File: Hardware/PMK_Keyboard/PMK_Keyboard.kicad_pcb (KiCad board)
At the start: 2 copper layers, 172 x 152 mm, 52 parts, among them IC1 SN74HC165PWR, IC2 SN74HC165PWR, IC3 SN74HC165PWR, IC4 SN74HC165PWR, IC5 SN74HC165PWR, IC7 ESP32-S2FH4, SW1 SW_Push, SW10 SW_Push, SW11 SW_Push, SW12 SW_Push, SW13 SW_Push, SW14 SW_Push, SW15 SW_Push, SW16 SW_Push, SW17 SW_Push, SW18 SW_Push, SW19 SW_Push, SW2 SW_Push, SW20 SW_Push, SW21 SW_Push, SW22 SW_Push, SW23 SW_Push, SW24 SW_Push, SW25 SW_Push, SW26 SW_Push, SW27 SW_Push, SW28 SW_Push, SW29 SW_Push, SW3 SW_Push, SW30 SW_Push, SW31 SW_Push, SW32 SW_Push, SW33 SW_Push, SW34 SW_Push, SW35 SW_Push, SW36 SW_Push, SW37 SW_Push, SW38 SW_Push, SW39 SW_Push, SW4 SW_Push, SW40 SW_Push, SW5 SW_Push, SW6 SW_Push, SW7 SW_Push, SW8 SW_Push, SW9 SW_Push

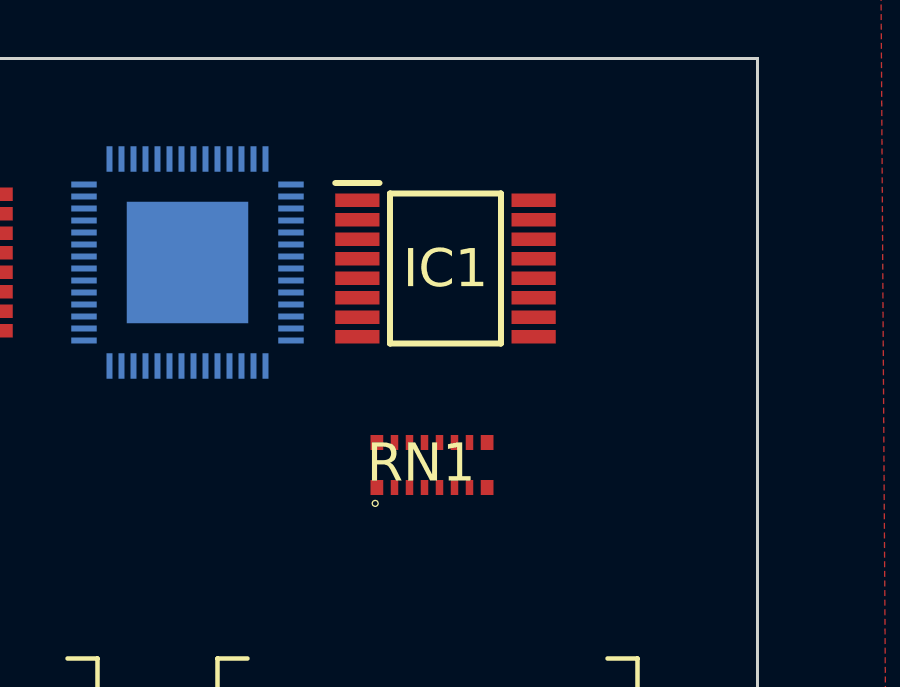
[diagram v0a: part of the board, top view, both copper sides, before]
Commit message: quick routing test
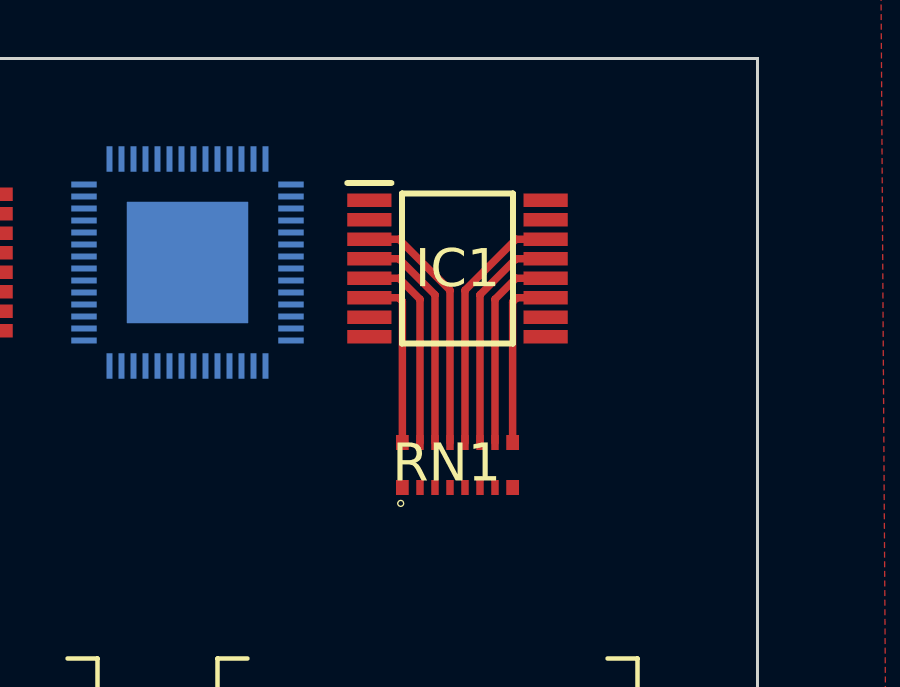
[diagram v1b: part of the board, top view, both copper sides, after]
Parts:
- moved RN1 0.85 mm to (145.0, 58.5)
- moved IC1 0.40 mm to (145.0, 52.0)
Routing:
- net /5: track 0.00 -> 8.47 mm
- net /4: track 0.00 -> 8.47 mm
- net /6: track 0.00 -> 7.61 mm
- net /3: track 0.00 -> 7.61 mm
- net /7: track 0.00 -> 6.75 mm
- net /2: track 0.00 -> 6.75 mm
- net /1: track 0.00 -> 5.86 mm
- net /8: track 0.00 -> 5.84 mm

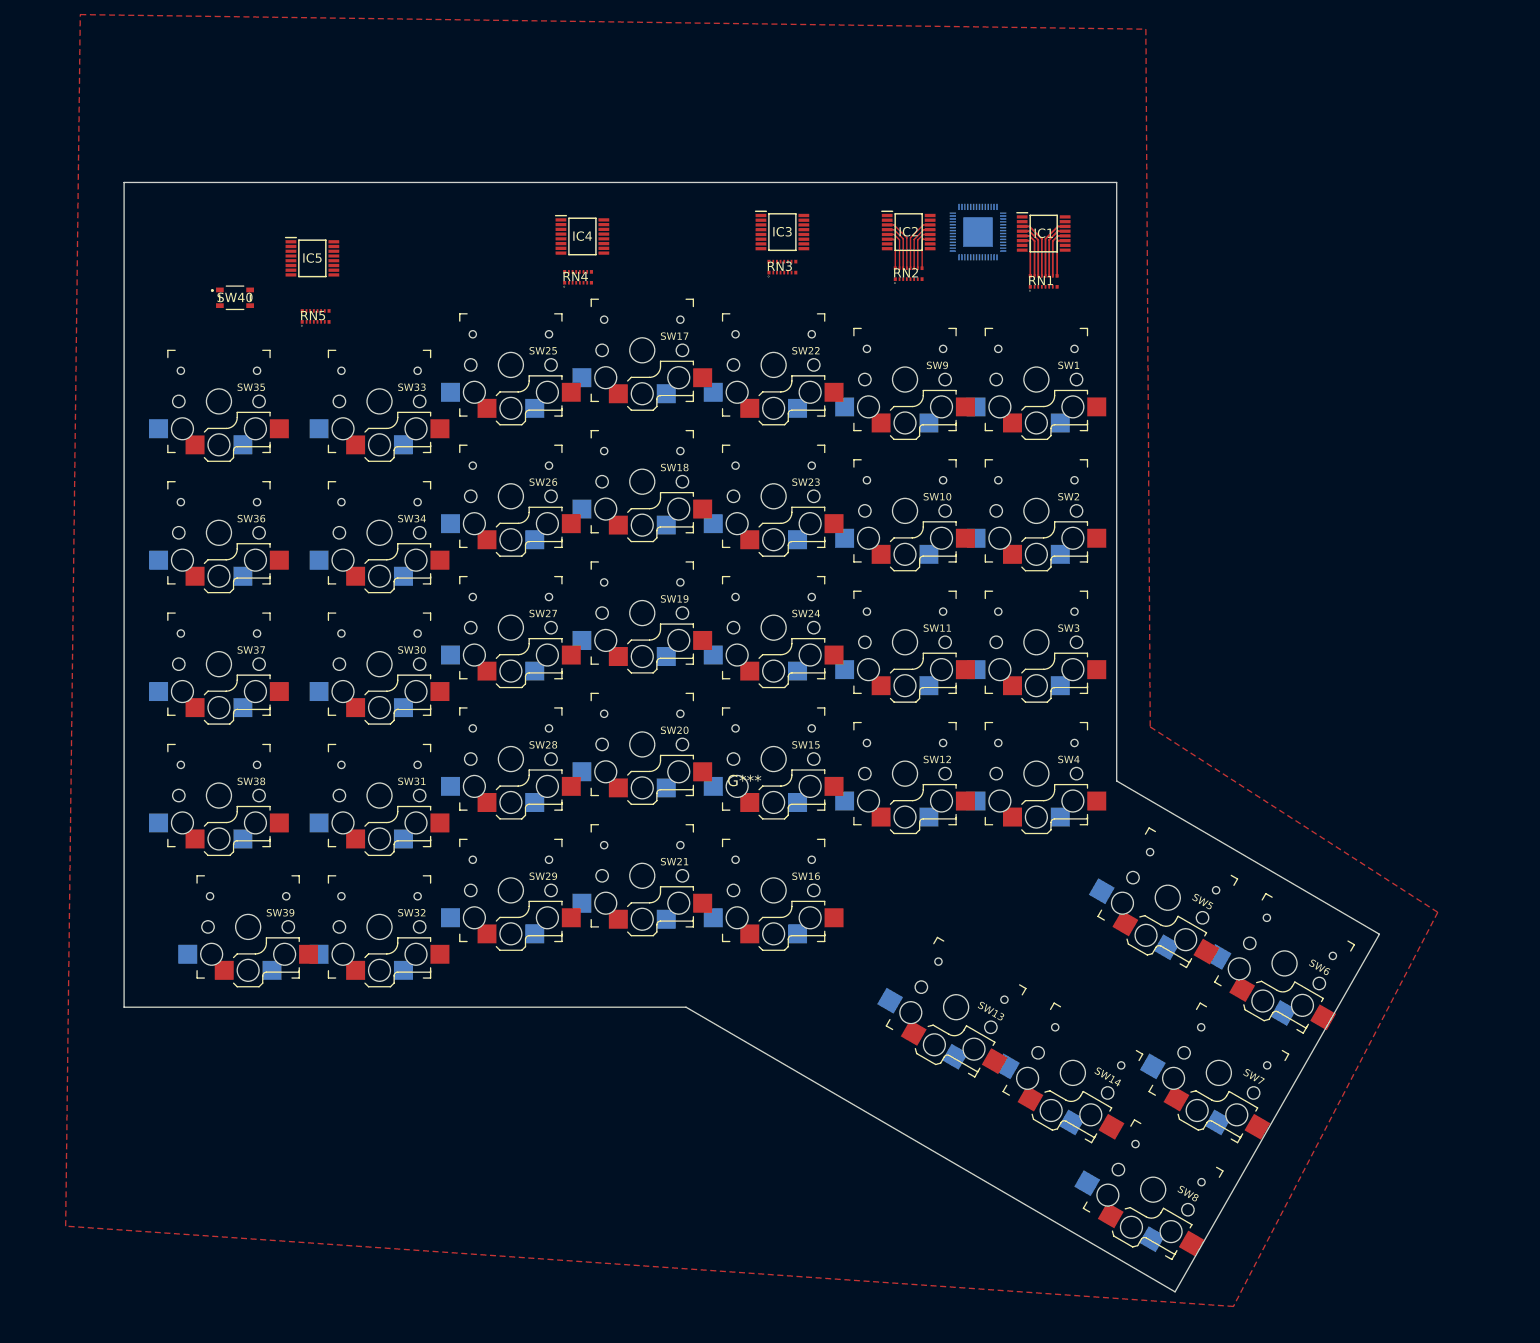
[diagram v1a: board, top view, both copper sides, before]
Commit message: Started routing
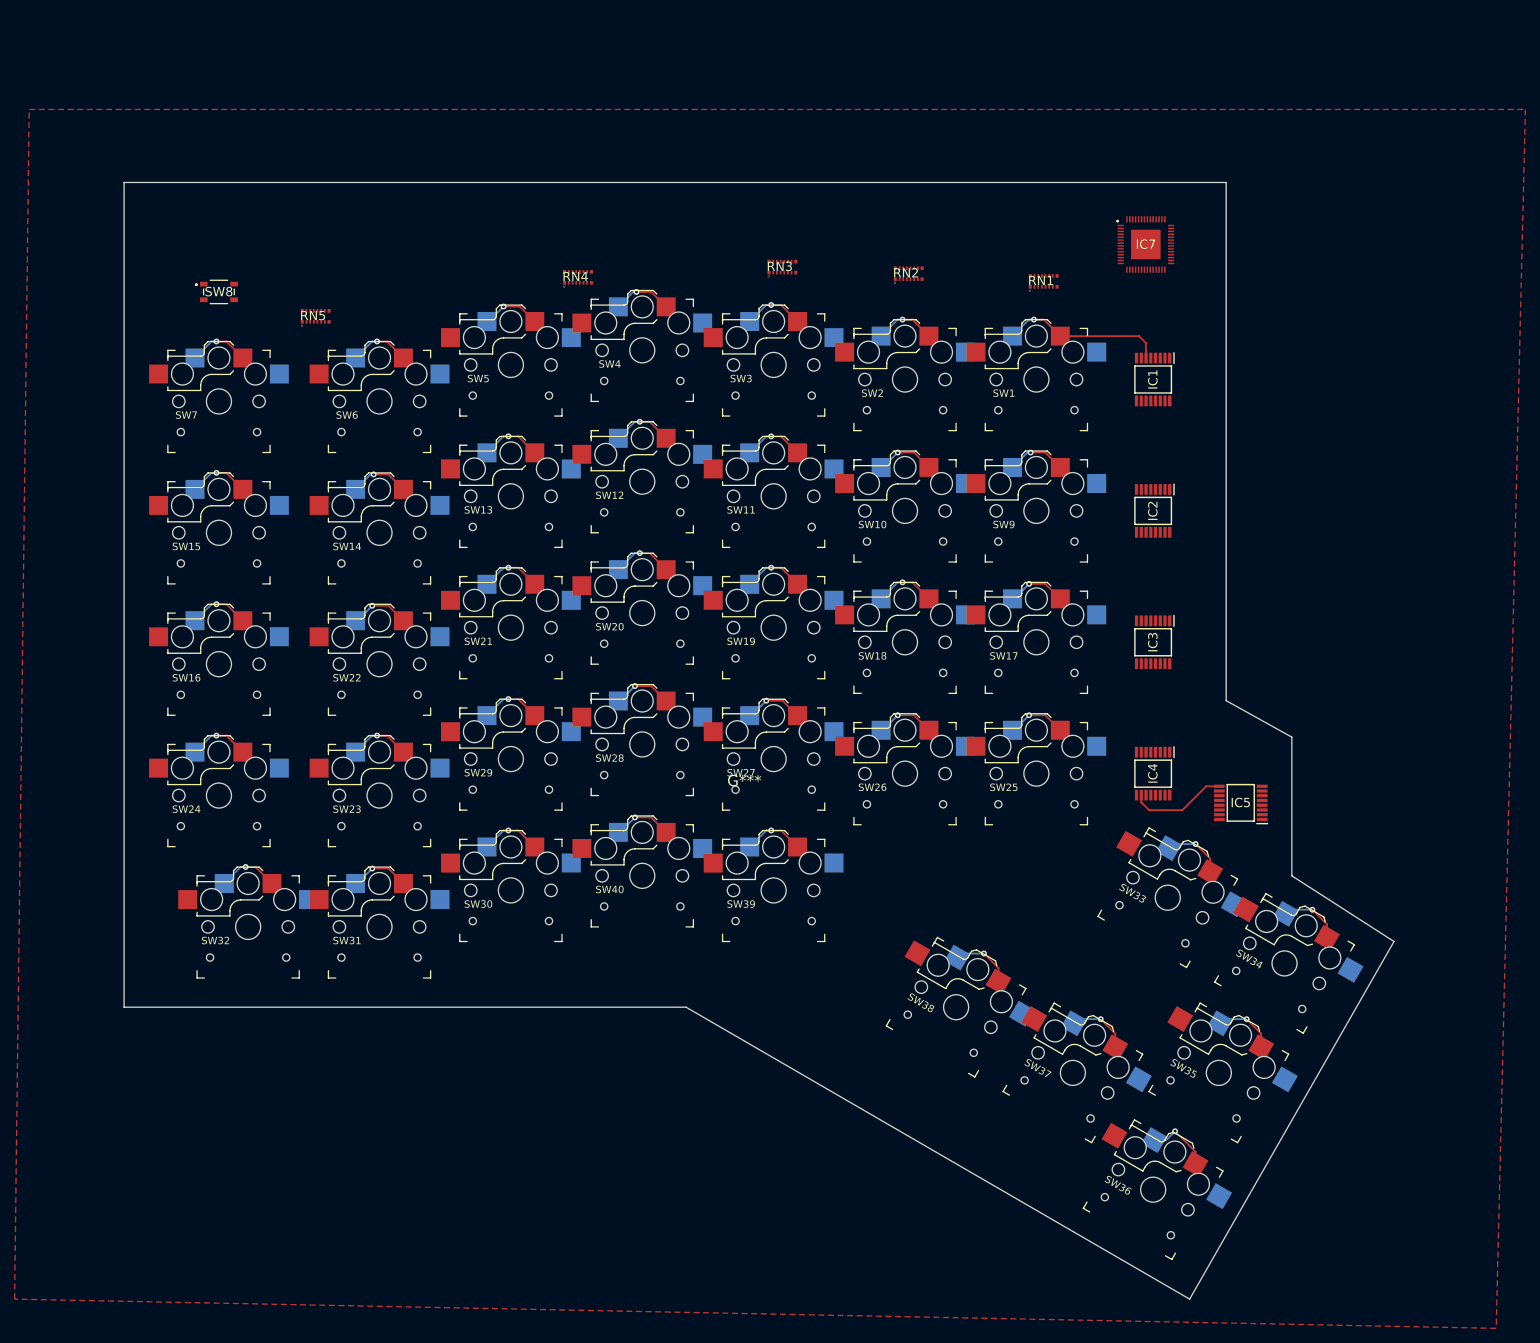
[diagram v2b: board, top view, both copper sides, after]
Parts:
- IC7: moved to F.Cu
- SW40: footprint Component_lib:SKRPABE010 -> Component_lib:Kailh_socket_PG1350_reversible
- SW8: footprint Component_lib:Kailh_socket_PG1350_reversible -> Component_lib:SKRPABE010
- moved SW8 177.5 mm to (32.0, 60.0), turned to 0 degrees
- moved SW35 165.0 mm to (169.0, 167.0), turned to 150 degrees
- moved SW7 165.0 mm to (32.0, 75.0), turned to 180 degrees
- moved SW36 156.5 mm to (160.0, 183.0), turned to 150 degrees
- moved IC5 147.5 mm to (172.0, 130.0), turned to 180 degrees
- moved SW6 146.0 mm to (54.0, 75.0), turned to 180 degrees
- moved SW34 137.3 mm to (178.0, 152.0), turned to 150 degrees
- moved SW37 129.7 mm to (149.0, 167.0), turned to 150 degrees
- moved SW33 127.6 mm to (162.0, 143.0), turned to 150 degrees
- moved SW14 120.4 mm to (54.0, 93.0), turned to 180 degrees
- moved SW5 115.9 mm to (72.0, 70.0), turned to 180 degrees
- moved IC4 107.4 mm to (160.0, 126.0), turned to -90 degrees
- moved SW38 105.1 mm to (133.0, 158.0), turned to 150 degrees
- moved SW40 96.9 mm to (90.0, 140.0), turned to 180 degrees
- moved SW13 92.8 mm to (72.0, 88.0), turned to 180 degrees
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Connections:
- SW1 pad 1: GND -> /1
- SW1 pad 2: /1 -> GND
- SW10 pad 1: GND -> /10
- SW10 pad 2: /10 -> GND
- SW11 pad 1: GND -> /11
- SW11 pad 2: /11 -> GND
- SW12 pad 1: GND -> /12
- SW12 pad 2: /12 -> GND
- SW13 pad 1: GND -> /13
- SW13 pad 2: /13 -> GND
- SW14 pad 1: GND -> /14
- SW14 pad 2: /14 -> GND
- SW15 pad 1: GND -> /15
- SW15 pad 2: /15 -> GND
- SW16 pad 1: GND -> /16
- SW16 pad 2: /16 -> GND
- SW17 pad 1: GND -> /17
- SW17 pad 2: /17 -> GND
- SW18 pad 1: GND -> /18
- SW18 pad 2: /18 -> GND
- SW19 pad 1: GND -> /19
- SW19 pad 2: /19 -> GND
- SW2 pad 1: GND -> /2
- SW2 pad 2: /2 -> GND
- SW20 pad 1: GND -> /20
- SW20 pad 2: /20 -> GND
- SW21 pad 1: GND -> /21
- SW21 pad 2: /21 -> GND
- SW22 pad 1: GND -> /22
- SW22 pad 2: /22 -> GND
- SW23 pad 1: GND -> /23
- SW23 pad 2: /23 -> GND
- SW24 pad 1: GND -> /24
- SW24 pad 2: /24 -> GND
- SW25 pad 1: GND -> /25
- SW25 pad 2: /25 -> GND
- SW26 pad 1: GND -> /26
- SW26 pad 2: /26 -> GND
- SW27 pad 1: GND -> /27
- SW27 pad 2: /27 -> GND
- SW28 pad 1: GND -> /28
- SW28 pad 2: /28 -> GND
- SW29 pad 1: GND -> /29
- SW29 pad 2: /29 -> GND
- SW3 pad 1: GND -> /3
- SW3 pad 2: /3 -> GND
- SW30 pad 1: GND -> /30
- SW30 pad 2: /30 -> GND
- SW31 pad 1: GND -> /31
- SW31 pad 2: /31 -> GND
- SW32 pad 1: GND -> /32
- SW32 pad 2: /32 -> GND
- SW33 pad 1: GND -> /33
- SW33 pad 2: /33 -> GND
- SW34 pad 1: GND -> /34
- SW34 pad 2: /34 -> GND
- SW35 pad 1: GND -> /35
- SW35 pad 2: /35 -> GND
- SW36 pad 1: GND -> /36
- SW36 pad 2: /36 -> GND
- SW37 pad 1: GND -> /37
- SW37 pad 2: /37 -> GND
- SW38 pad 1: GND -> /38
- SW38 pad 2: /38 -> GND
- SW39 pad 1: GND -> /39
- SW39 pad 2: /39 -> GND
- SW4 pad 1: GND -> /4
- SW4 pad 2: /4 -> GND
- SW40 pad 1: GND -> /40
- SW40 pad 2: /40 -> GND
- SW5 pad 1: GND -> /5
- SW5 pad 2: /5 -> GND
- SW6 pad 1: GND -> /6
- SW6 pad 2: /6 -> GND
- SW7 pad 1: GND -> /7
- SW7 pad 2: /7 -> GND
- SW8 pad 1: GND -> /8
- SW8 pad 2: /8 -> GND
- SW9 pad 1: GND -> /9
- SW9 pad 2: /9 -> GND
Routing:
- net /1: track 5.86 -> 22.6 mm, vias 0 -> 1
- net /4-5: track 0.00 -> 13.5 mm
- net /36: track 0.00 -> 9.01 mm, vias 0 -> 1
- net /38: track 0.00 -> 8.58 mm, vias 0 -> 1
- net /37: track 0.00 -> 8.58 mm, vias 0 -> 1
- net /35: track 0.00 -> 8.58 mm, vias 0 -> 1
- net /34: track 0.00 -> 8.58 mm, vias 0 -> 1
- net /33: track 0.00 -> 8.58 mm, vias 0 -> 1
- net /39: track 0.00 -> 8.42 mm, vias 0 -> 1
- net /30: track 0.00 -> 8.42 mm, vias 0 -> 1
- net /32: track 0.00 -> 8.42 mm, vias 0 -> 1
- net /29: track 0.00 -> 8.42 mm, vias 0 -> 1
- net /21: track 0.00 -> 8.42 mm, vias 0 -> 1
- net /20: track 0.00 -> 8.42 mm, vias 0 -> 1
- net /19: track 0.00 -> 8.42 mm, vias 0 -> 1
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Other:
- board size 172 x 152 mm -> 174 x 153 mm
